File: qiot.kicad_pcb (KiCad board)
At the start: 4 copper layers, 186.1 x 116.9 mm, 299 parts, among them J1 Conn_01x05, J10 Conn_01x06, J11 TE_4-1734592-0, J12 Barrel_Jack, J13 CELLS1, J14 CELLS1, J15 Conn_01x03, J16 Conn_01x03, J17 PWRSWITCH, J18 Conn_01x02, J19 EN, J2 Conn_01x03, J20 Conn_01x03, J21 PGOOD, J22 Conn_01x03, J23 Conn_01x04, J24 Conn_01x04, J25 Conn_01x04, J26 TYPE-C-31-M-12, J27 Conn_01x03, J28 Conn_01x03, J29 EnUSB, J3 TYPE-C-31-M-12, J30 BAMBANG_CONNECTOR, J4 Conn_01x02, J5 Conn_01x02, J6 BATT2_jmp, J7 BATT2_jmp, J8 BATT1_jmp, J9 Conn_02x03_Odd_Even, Q1 PMBT2222A, Q10 IRLZ44NSTRL(UMW), Q2 PMBT2222A, Q3 PMBT2222A, Q4 IRLZ44NSTRL(UMW), Q5 IRLZ44NSTRL(UMW), Q6 2N7002, Q7 BSS223PW, Q8 PMBT2222A, Q9 IRLZ44NSTRL(UMW), SW1 SW_SPDT_312, U1 UM803RS, U10 TLV62130, U11 DRV8825, U12 FC41D, U13 TLV62130, U14 PCA9539PW_118, U2 MIMXRT1011DAE5A, U3 TS5A3159DBVR, U4 W25Q128JVS, U5 MAX17320G20+T, U6 LTC4162EUFD, U7 TLV62130, U8 TLV62130, U9 MAX42402AFLB+, Y1 24MHz, Y2 32.768KHz

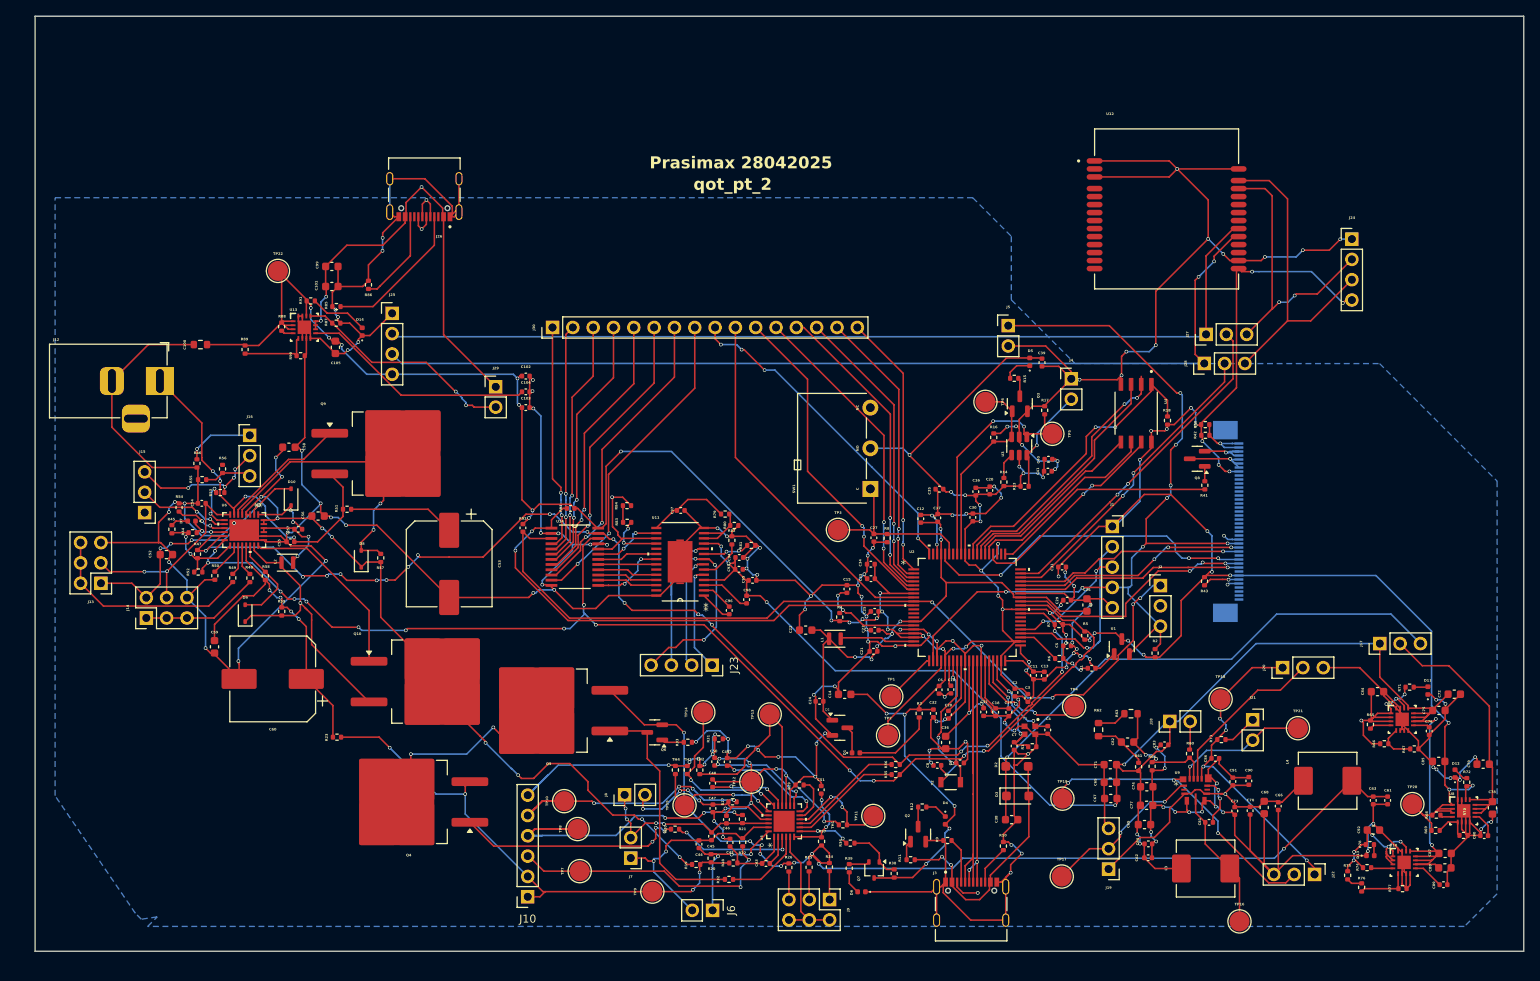
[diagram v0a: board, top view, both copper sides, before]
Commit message: gema
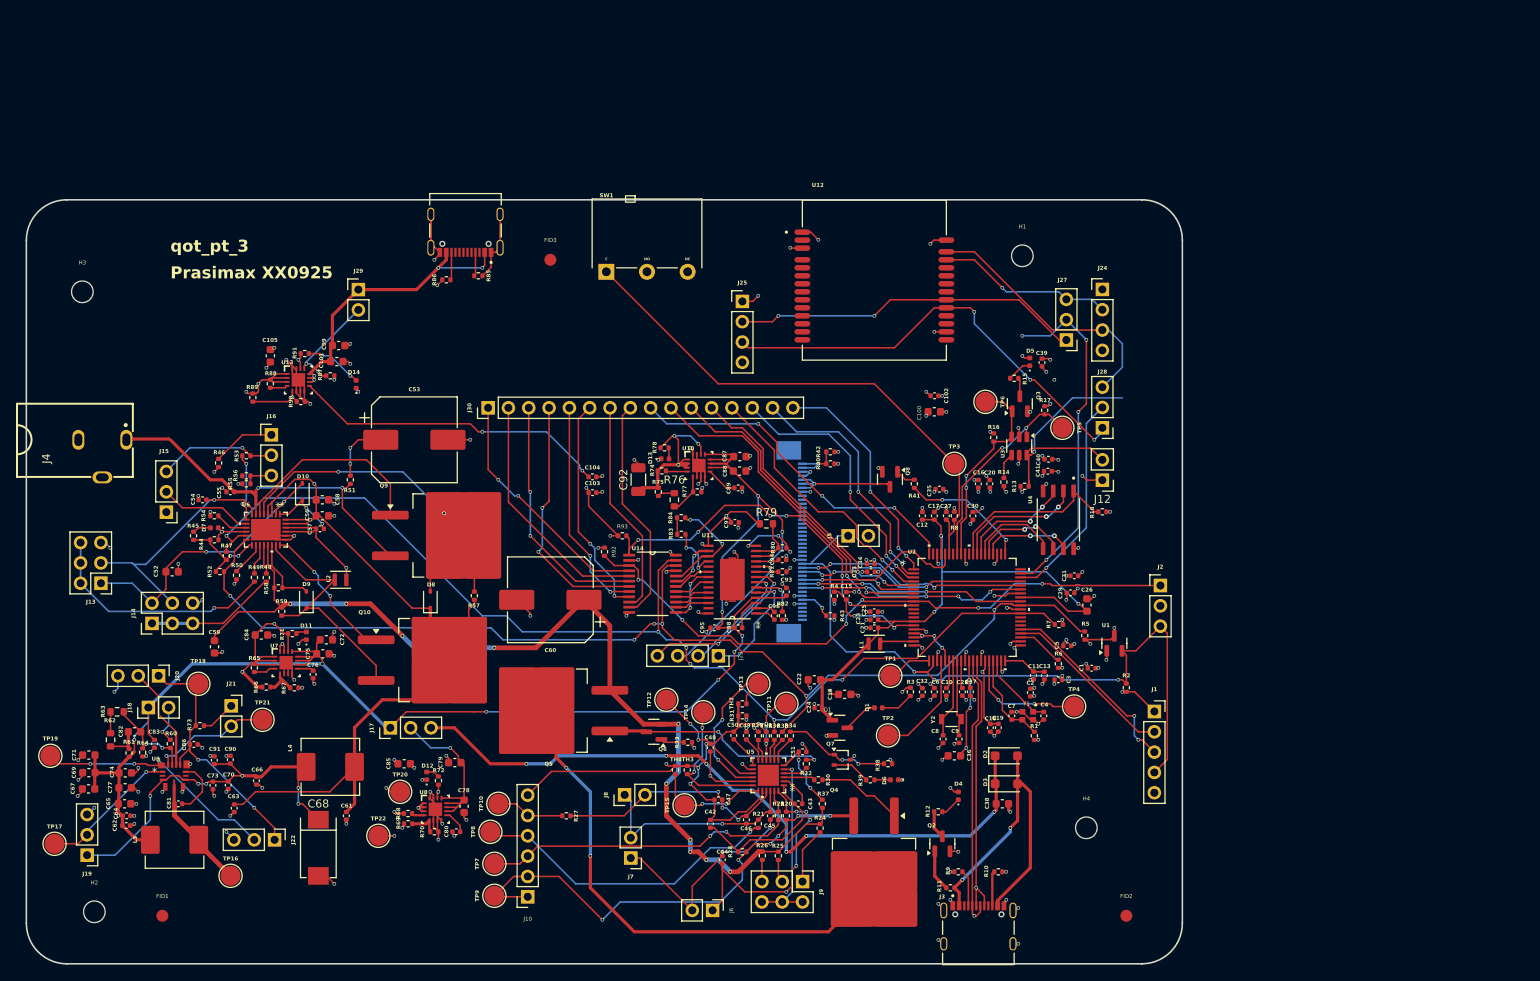
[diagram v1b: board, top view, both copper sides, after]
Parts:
- removed R19, R23: 0, Resistor_SMD:R_0402_1005Metric
- added FID1: Fiducial, Fiducial:Fiducial_1.5mm_Mask3mm, F.Cu at (36.5, 152.5)
- added FID2: Fiducial, Fiducial:Fiducial_1.5mm_Mask3mm, F.Cu at (157.0, 152.5)
- added FID3: Fiducial, Fiducial:Fiducial_1.5mm_Mask3mm, F.Cu at (85.0, 70.5)
- added H1: MountingHole, MountingHole:MountingHole_2.7mm_M2.5, F.Cu at (144.0, 70.0)
- added H2: MountingHole, MountingHole:MountingHole_2.7mm_M2.5, F.Cu at (28.0, 152.0)
- added H3: MountingHole, MountingHole:MountingHole_2.7mm_M2.5, F.Cu at (26.5, 74.5)
- added H4: MountingHole, MountingHole:MountingHole_2.7mm_M2.5, F.Cu at (152.0, 141.5)
- C1, C41: value 1.0uF -> 1uF
- C10, C11, C12, C15, C17, C19, C21, C3, C5, C6: value 0.22uF -> 220nF
- C100: footprint Resistor_SMD:R_0603_1608Metric -> Capacitor_SMD:C_0603_1608Metric
- C101, C72, C75, C78, C79, C87, C88, C99: value 10u -> 10uF
- C104, C76, C80, C89: value 1n -> 1nF
- C105, C84, C85: value 47u -> 47uF
- C14, C22: value 22uF_0603 -> 22uF
- C16: value 4.7uF_0402 -> 4.7uF
- C20, C24, C25, C27: value 0.22uF_0402 -> 220nF
- C28: value 1.0uF_0402 -> 1uF
- C36: value 10uF_0603 -> 10uF
- C37: value 100nF_0402 -> 100nF
- C42, C55, C62, C63, C64, C66, C73, C81, C83, C90, C94, C95, C98: value 0.1uF -> 100nF
- C43, C48, C50, C97: value 0.47uF -> 470nF
- C44, C45, C46, C47, C49, C51: value 0.01uF -> 10nF
- C57: value 0.022uF -> 22nF
- C68: footprint Capacitor_SMD:C_0603_1608Metric -> footprints:CAP-SMD_L7.3-W4.3-R-RD
- C92: value 47u -> 47uF; footprint Capacitor_SMD:C_0603_1608Metric -> Capacitor_SMD:C_1206_3216Metric
- J12: value Barrel_Jack -> Conn_01x02; footprint Connector_BarrelJack:BarrelJack_Horizontal -> Connector_PinHeader_2.54mm:PinHeader_1x02_P2.54mm_Vertical
- J4: value Conn_01x02 -> PJ-102AH; footprint Connector_PinHeader_2.54mm:PinHeader_1x02_P2.54mm_Vertical -> footprints:DC-IN-TH_PJ-102AH
- R13, R16, R17, R38, R48, R49: value 100k -> 100K
- R18, R33: value 10k -> 10K
- R31: value 0.005 -> 0.05
- R37, R42: value 1k -> 1K
- R4: value 30k -> 30K
- R50: value 10.0k -> 10K
- R54: value 63.4k -> 63.4K
- R65, R68, R74, R88: value 4.7k -> 4.7K
- R69, R89: value 47k -> 47K
- R70, R90: value 15k -> 15K
- R71, R72, R78, R91: value 2.49k -> 2.49K
- R76, R79: footprint Resistor_SMD:R_0402_1005Metric -> Resistor_SMD:R_0603_1608Metric
- R92, R93: footprint Capacitor_SMD:C_0402_1005Metric -> Resistor_SMD:R_0402_1005Metric
- moved C63 142.4 mm to (45.5, 139.1)
- moved C72 141.2 mm to (57.0, 118.0)
- moved J20 140.5 mm to (36.0, 122.5), turned to -90 degrees
- moved D11 140.4 mm to (54.5, 117.5)
- moved R67 140.2 mm to (53.0, 124.0)
- moved R66 139.9 mm to (49.5, 123.9)
- moved R71 139.8 mm to (52.7, 117.2)
- moved C76 139.7 mm to (55.4, 122.3)
- moved C84 139.7 mm to (48.9, 117.4)
- moved C75 139.7 mm to (56.6, 119.8)
- moved R65 139.7 mm to (48.0, 121.5)
- moved U7 139.7 mm to (52.0, 120.9)
- moved C61 130.2 mm to (59.5, 140.0)
- moved J22 130.1 mm to (50.5, 143.0)
- moved TP21 129.4 mm to (49.0, 128.0)
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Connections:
- C61 pad 1: SYSP -> VOUT_BATCHG
- C63 pad 1: SYSP -> VOUT_BATCHG
- J12 pad 1: VIN_CHG -> SYSN
- J12 pad 2: SYSN -> /03_BOOTLOADER/BOOT_SEL
- J4 pad 1: SYSN -> VIN_CHG
- J4 pad 2: /03_BOOTLOADER/BOOT_SEL -> unconnected-(J4-Pad2)
- L4 pad 1: SYSP -> VOUT_BATCHG
- Q5 pad 3: SYSP -> BATSENS_CHG
- Q6 pad 2: SYSP -> BATSENS_CHG
- R24 pad 1: SYSP -> BATSENS_CHG
- R25 pad 1: SYSP -> BATSENS_CHG
- R26 pad 1: SYSP -> BATSENS_CHG
- R37 pad 1: SYSP -> BATSENS_CHG
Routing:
- net SYSN: track 1009.9 -> 241.4 mm, vias 132 -> 177
- net 3P3V: track 548.1 -> 94.5 mm, vias 63 -> 66
- net SYSP: track 127.7 -> 0.00 mm, vias 9 -> 0
- net BATSENS_CHG: track 40.1 -> 124.4 mm, vias 4 -> 10
- net FC41D_UART_TX_MAIN: track 117.3 -> 43.7 mm, vias 0 -> 2
- net FC41D_UART_RX_MAIN: track 121.0 -> 56.0 mm, vias 2 -> 3
- net Net-(SW1-B): track 21.8 -> 67.7 mm
- net Net-(Q4-D): track 21.7 -> 57.3 mm
- net /04_bateryMon/BATT1: track 35.2 -> 8.61 mm, vias 4 -> 0
- net ~{RESET_PCA9539PW}: track 105.7 -> 79.4 mm, vias 4 -> 6
- net VSYS_USB: track 68.5 -> 88.9 mm, vias 1 -> 6
- net LCD_DC: track 42.1 -> 21.7 mm, vias 3 -> 1
- net JTAG_RESET: track 109.9 -> 91.0 mm, vias 9 -> 3
- net /03_BOOTLOADER/BOOT_SEL: track 13.3 -> 31.2 mm
- net /10_wifi/VBUS_USB: track 55.1 -> 37.5 mm, vias 3 -> 4
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- removed copper zone on B.Cu, net VMM_motor
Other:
- board size 186.1 x 116.9 mm -> 144.5 x 95.5 mm
- board text added: "Prasimax XX0925"
- board text added: "qot_pt_3"
- board text removed: "Prasimax 28042025"
- board text removed: "qot_pt_2"
